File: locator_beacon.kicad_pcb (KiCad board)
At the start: 2 copper layers, 50.9 x 20.8 mm, 35 parts, among them J1 Conn_01x02, J2 Conn_01x02, Q1 DMN6140, Q2 DMN6140, Q3 DMN6140, Q4 DMN6140, U1 MC34063AD, U13 Pico, U3 MIC4606

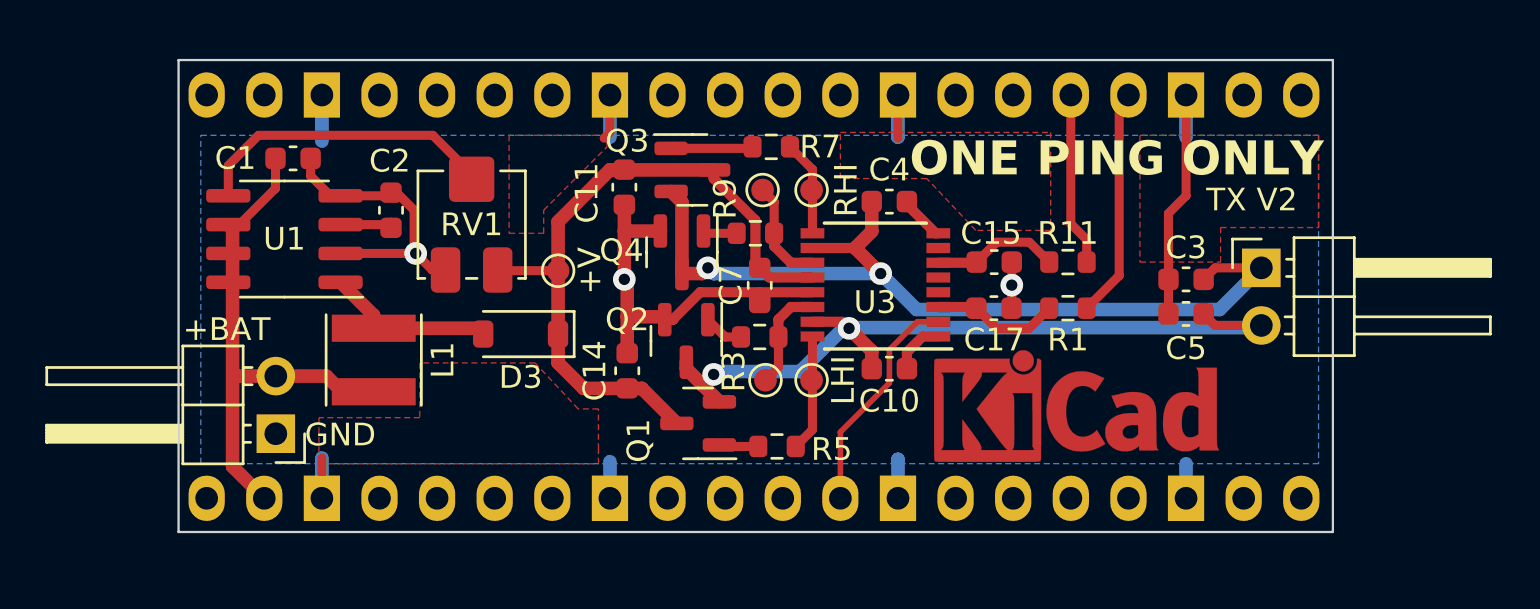
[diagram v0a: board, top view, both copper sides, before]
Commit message: changes
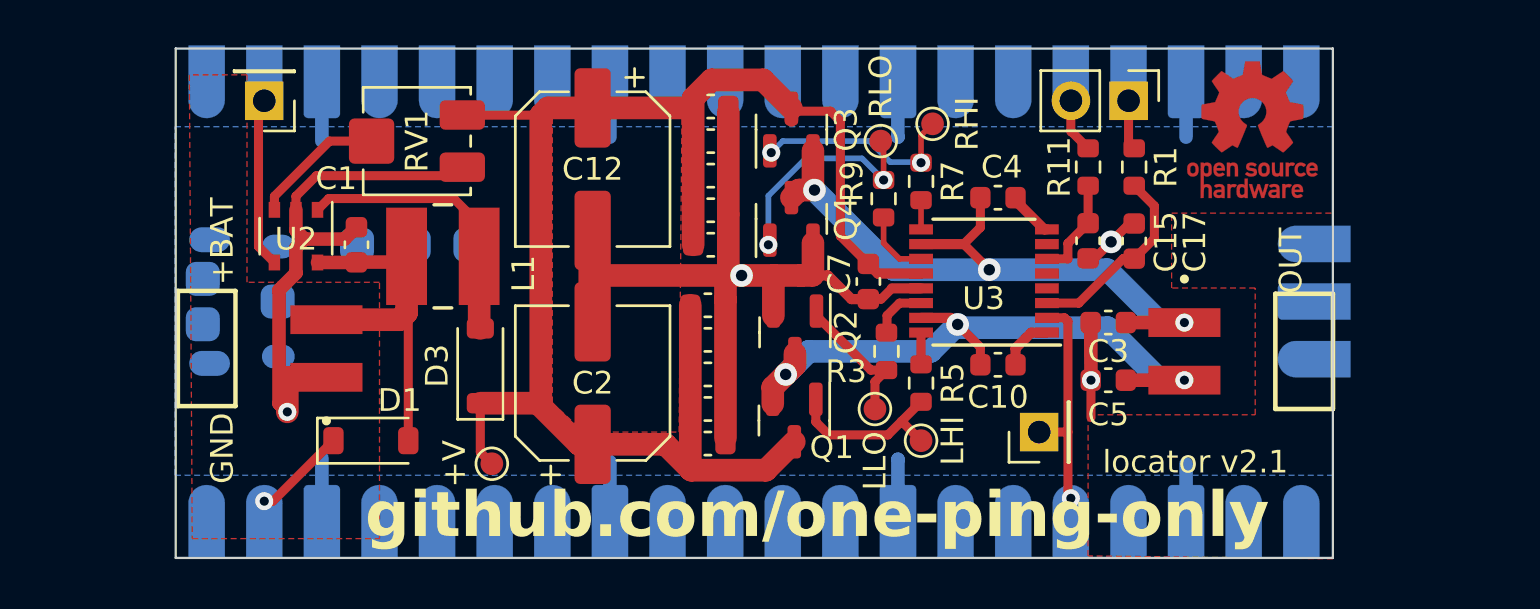
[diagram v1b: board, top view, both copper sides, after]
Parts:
- removed REF**: KiCad-Logo_5mm_Copper, Symbol:KiCad-Logo_5mm_Copper
- removed U1: MC34063AD, Package_SO:SOIC-8_3.9x4.9mm_P1.27mm
- added C12: C, Capacitor_SMD:CP_Elec_6.3x7.7, F.Cu at (136.1, 72.6)
- added C13: 10u, Capacitor_SMD:C_0603_1608Metric, F.Cu at (141.2, 81.7)
- added C16: 10u, Capacitor_SMD:C_0603_1608Metric, F.Cu at (141.2, 83.2)
- added C18: 10u, Capacitor_SMD:C_0603_1608Metric, F.Cu at (141.2, 80.1)
- added C19: 10u, Capacitor_SMD:C_0603_1608Metric, F.Cu at (141.2, 78.6)
- added C20: 10u, Capacitor_SMD:C_0603_1608Metric, F.Cu at (141.4, 71.4)
- added C6: 10u, Capacitor_SMD:C_0603_1608Metric, F.Cu at (141.2, 84.7)
- added C8: 10u, Capacitor_SMD:C_0603_1608Metric, F.Cu at (141.4, 69.8)
- added C9: 10u, Capacitor_SMD:C_0603_1608Metric, F.Cu at (141.4, 72.9)
- added D1: DSS16U, Diode_SMD:D_SOD-123, F.Cu at (126.4, 84.6)
- added J3: Conn_01x01, Connector_PinHeader_2.54mm:PinHeader_1x01_P2.54mm_Vertical, F.Cu at (155.8, 84.2)
- added J4: OSHW logo, Symbol:OSHW-Logo_5.7x6mm_Copper, F.Cu at (165.2, 70.9)
- added J6: Conn_01x01, Connector_PinHeader_2.54mm:PinHeader_1x01_P2.54mm_Vertical, F.Cu at (121.7, 69.6)
- added J7: Conn_01x02, Connector_PinHeader_2.54mm:PinHeader_1x02_P2.54mm_Vertical, F.Cu at (159.8, 69.6)
- added U2: MIC2288, Package_SO:TSOP-5_1.65x3.05mm_P0.95mm, F.Cu at (123.1, 75.6)
- C2: value 1.5n -> C; footprint Capacitor_SMD:C_0603_1608Metric -> Capacitor_SMD:CP_Elec_6.3x7.7
- J1, J2: footprint Connector_PinHeader_2.54mm:PinHeader_1x02_P2.54mm_Horizontal -> custom:SAMTEC_TSM-102-01-L-SH
- L1: footprint Inductor_SMD:L_Taiyo-Yuden_MD-4040 -> custom:IND_357100_WRE
- U13: footprint custom:rp_pico -> custom:RPi_pico
- moved C2 11.7 mm to (136.1, 82.0)
- moved TP1 9.00 mm to (131.7, 85.6)
- moved C14 7.98 mm to (141.4, 74.4), turned to 0 degrees
- moved R5 6.94 mm to (150.6, 82.0), turned to 90 degrees
- moved R1 6.87 mm to (160.0, 72.5), turned to 90 degrees
- moved C17 6.86 mm to (160.0, 75.8), turned to 90 degrees
- moved R7 6.78 mm to (150.6, 73.2), turned to 90 degrees
- moved TP7 6.08 mm to (151.1, 70.6)
- moved R9 5.85 mm to (149.0, 73.9), turned to 90 degrees
- moved TP6 5.64 mm to (148.8, 71.4)
- moved R3 5.62 mm to (149.1, 80.6), turned to 90 degrees
- moved TP2 5.51 mm to (150.6, 84.6)
- moved L1 5.49 mm to (129.5, 76.5), turned to 0 degrees
- moved Q4 5.05 mm to (144.9, 74.8), turned to 90 degrees
- moved TP4 4.99 mm to (148.6, 83.2)
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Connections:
- C2 pad 1: Net-(U1-TC) -> Vdrive
- TP2 pad 1: /amplifier/L_HI -> Net-(Q1-G)
- TP4 pad 1: /amplifier/L_LO -> Net-(Q2-G)
- TP6 pad 1: /amplifier/R_LO -> Net-(Q4-G)
- TP7 pad 1: /amplifier/R_HI -> Net-(Q3-G)
- U13 pad 2: unconnected-(U13-GPIO1-Pad2) -> /power/EN
- U13 pad 25: unconnected-(U13-GPIO19-Pad25) -> /amplifier/EN
- U13 pad 29: /amplifier/EN -> unconnected-(U13-GPIO22-Pad29)
- U13 pad 39: +BATT -> Net-(D1-K)
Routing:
- net Vdrive: track 31.2 -> 72.7 mm
- net GND: track 63.4 -> 83.9 mm, vias 3 -> 4
- net /amplifier/OUT_B: track 39.4 -> 29.7 mm, vias 2 -> 3
- net Net-(Q4-G): track 1.51 -> 10.1 mm, vias 0 -> 2
- net +BATT: track 23.8 -> 15.9 mm
- net /amplifier/SIG_IN: track 10.5 -> 2.58 mm
- net /power/EN: track 0.00 -> 7.78 mm
- net Net-(U2-FB): track 13.5 -> 5.89 mm
- net /amplifier/OUT_A: track 35.1 -> 28.9 mm, vias 2 -> 3
- net Net-(Q1-G): track 1.74 -> 7.49 mm
- net Net-(Q3-G): track 3.62 -> 9.13 mm, vias 0 -> 2
- net Net-(D3-A): track 7.48 -> 12.4 mm
- net /amplifier/~{SIG_IN}: track 7.66 -> 2.90 mm
- net Net-(Q2-G): track 1.78 -> 6.00 mm
- net Net-(D1-K): track 0.00 -> 4.15 mm, vias 0 -> 1
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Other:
- board size 50.9 x 20.8 mm -> 51 x 22.5 mm
- board text added: "OUT"
- board text added: "github.com/one-ping-only"
- board text added: "locator v2.1"
- board text removed: "ONE PING ONLY"
- board text removed: "TX V2"
